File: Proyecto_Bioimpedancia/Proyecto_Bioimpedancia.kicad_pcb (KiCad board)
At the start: 2 copper layers, 55 parts, among them J1 Jumper_Calibration, J2 Jumper, J3 Jumper, J4 Jumper, P1 CONN_01X03, P2 CONN_01X02, P3 CONN_01X02, P4 CONN_01X01, P5 CONN_01X01, P6 CONN_01X02, SW1 SW_PUSH, U1 AD8606, U2 ADG819, U3 Atmega328PA, U4 KC5032A_CM, U5 ADP3303, Y1 AMB3_16M

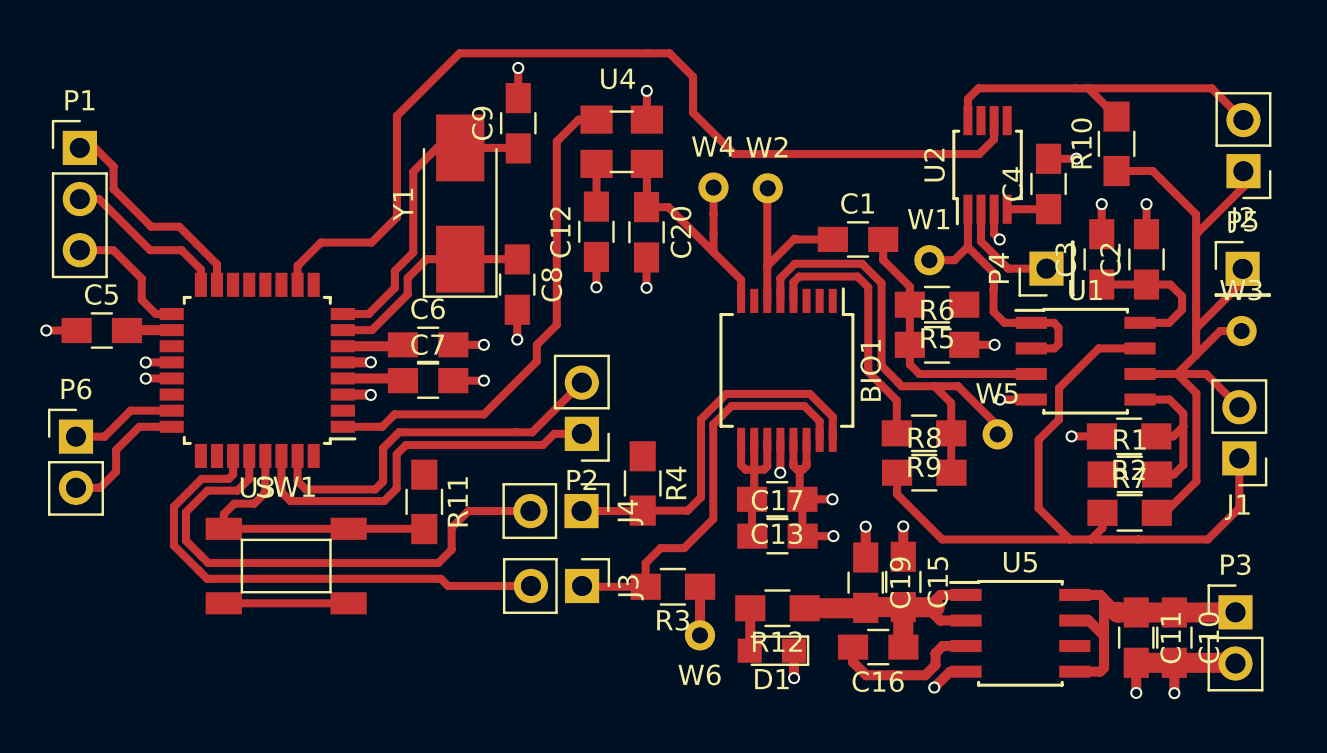
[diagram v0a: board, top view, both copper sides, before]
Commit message: PCB Final
Falta ultima revisión Esquematico
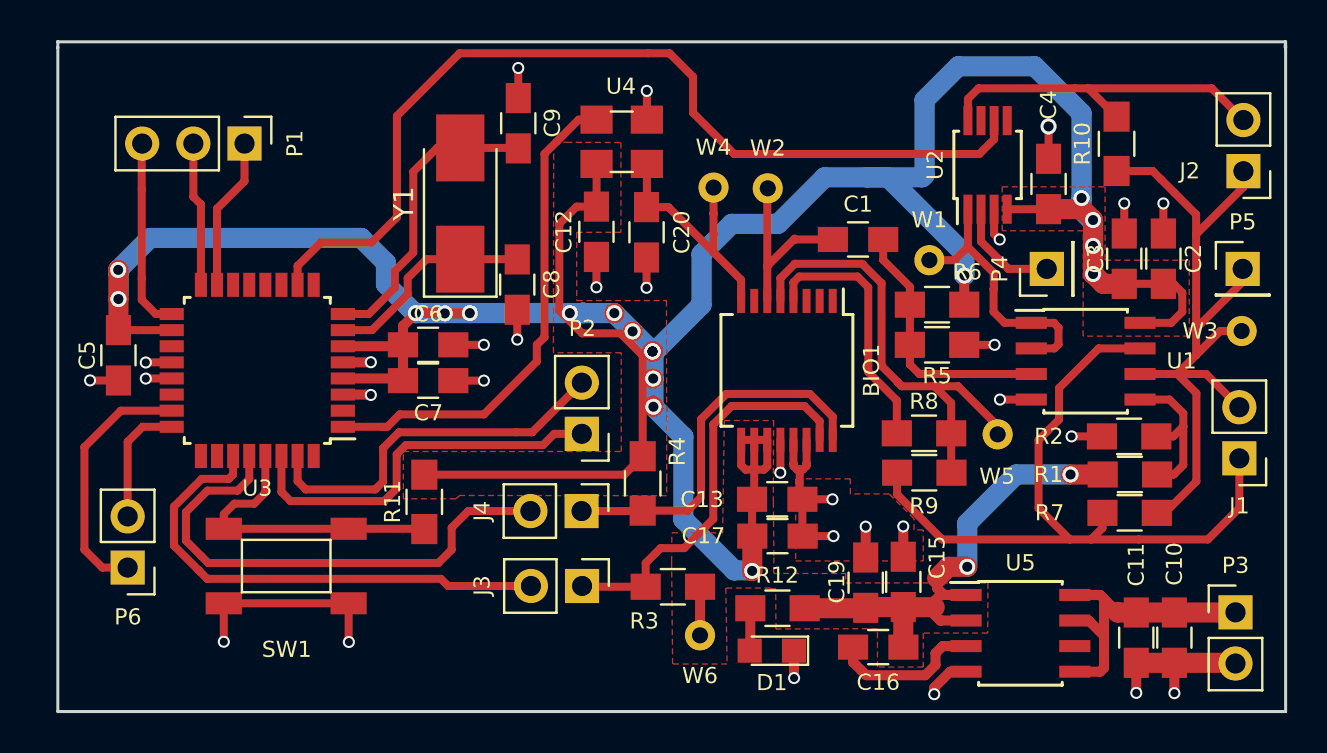
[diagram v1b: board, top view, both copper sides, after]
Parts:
- moved P1 8.18 mm to (185.5, 57.0), turned to 270 degrees
- moved P6 6.99 mm to (179.7, 78.1), turned to 180 degrees
- moved C5 1.48 mm to (179.2, 67.5), turned to 90 degrees
- moved C3 1.12 mm to (229.1, 62.7)
- moved C2 0.84 mm to (231.1, 62.7)
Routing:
- net /3V3: track 44.0 -> 199.0 mm, vias 0 -> 20
- net /ADC0: track 5.29 -> 12.7 mm
- net /AGND: track 59.8 -> 64.1 mm, vias 28 -> 30
- net /MOSI: track 10.9 -> 7.58 mm
- net /SCK: track 6.49 -> 9.55 mm
- net /MISO: track 8.22 -> 7.17 mm
- added copper zone on F.Cu, net /3V3
- added copper zone on B.Cu, net /AGND
- added copper zone on F.Cu, net /AGND
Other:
- board outline added: 61 x 33.3 mm
